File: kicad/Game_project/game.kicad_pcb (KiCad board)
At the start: 2 copper layers, 149.8 x 99.6 mm, 33 parts, among them J3 Conn_01x05_Socket, J4 Conn_01x05_Socket, J5 USB_B, J6 ISP header, U1 MAX7219, U10 HDSP-7403, U2 ATmega328P-P, U5 HDSP-7403, U6 HDSP-7403, U7 HDSP-7403, U8 HDSP-7403, U9 HDSP-7403

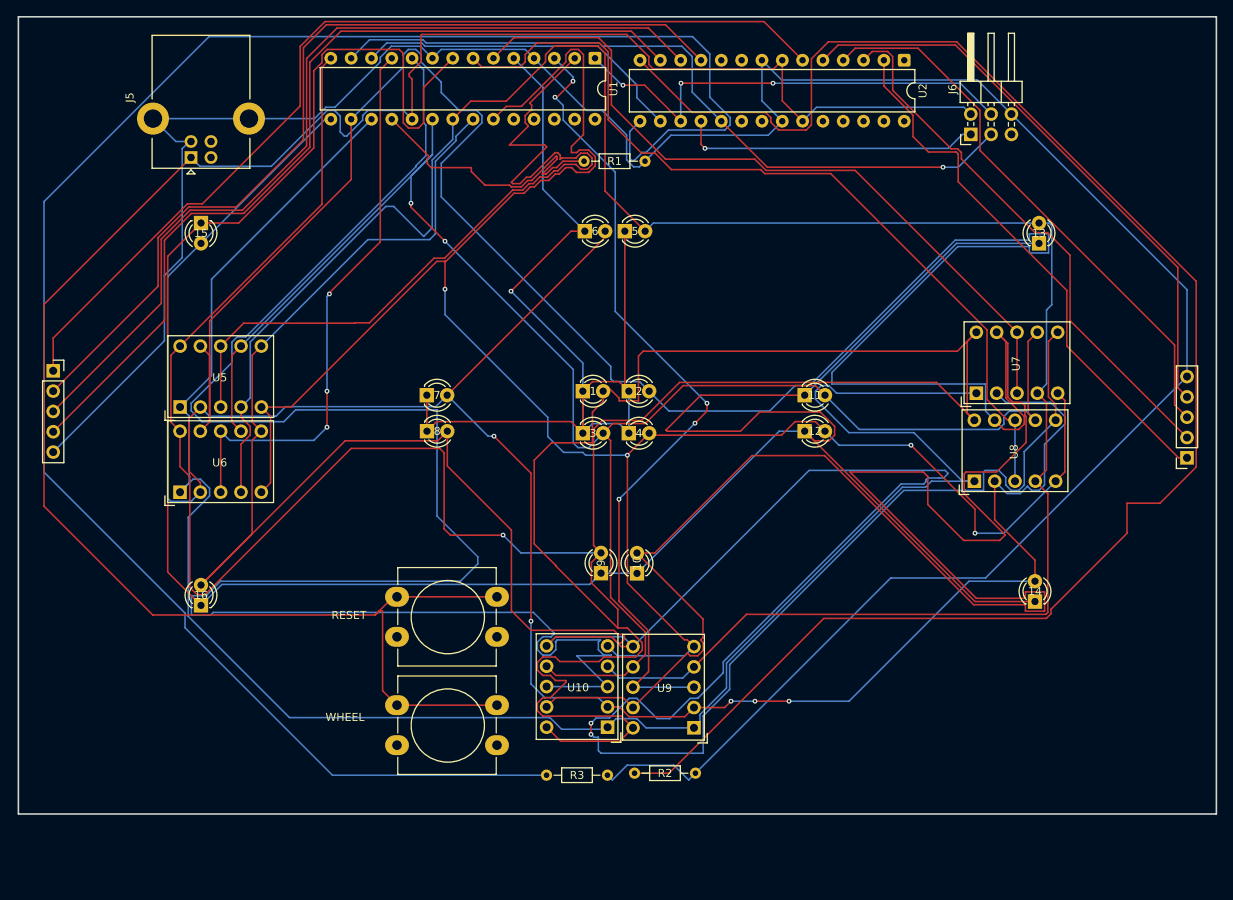
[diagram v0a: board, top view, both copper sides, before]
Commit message: orded
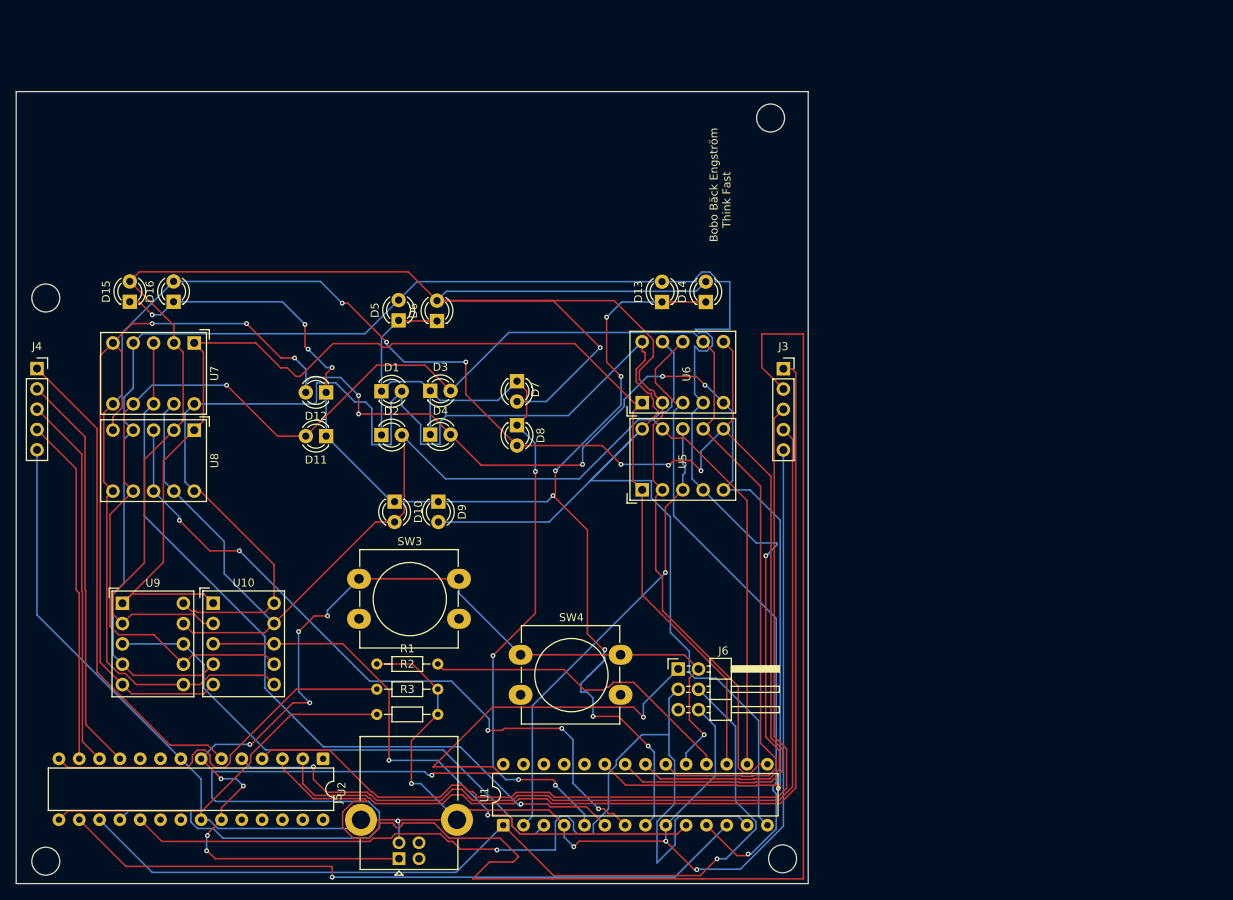
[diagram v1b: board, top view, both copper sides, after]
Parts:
- removed 1, 10, 11, 12, 13, 14, 15, 16, 2, 3, 4, 5, 6, 7, 8, 9: LED, LED_THT:LED_D3.0mm_Clear
- removed RESET, WHEEL: SW_pin12, Button_Switch_THT:SW_PUSH-12mm_Wuerth-430476085716
- added D1: LED, LED_THT:LED_D3.0mm_Clear, F.Cu at (145.6, 97.3)
- added D10: LED, LED_THT:LED_D3.0mm_Clear, F.Cu at (147.2, 111.1)
- added D11: LED, LED_THT:LED_D3.0mm_Clear, F.Cu at (138.6, 102.9)
- added D12: LED, LED_THT:LED_D3.0mm_Clear, F.Cu at (138.6, 97.4)
- added D13: LED, LED_THT:LED_D3.0mm_Clear, F.Cu at (180.6, 86.1)
- added D14: LED, LED_THT:LED_D3.0mm_Clear, F.Cu at (186.1, 86.1)
- added D15: LED, LED_THT:LED_D3.0mm_Clear, F.Cu at (114.1, 86.1)
- added D16: LED, LED_THT:LED_D3.0mm_Clear, F.Cu at (119.6, 86.1)
- added D2: LED, LED_THT:LED_D3.0mm_Clear, F.Cu at (145.6, 102.7)
- added D3: LED, LED_THT:LED_D3.0mm_Clear, F.Cu at (151.7, 97.2)
- added D4: LED, LED_THT:LED_D3.0mm_Clear, F.Cu at (151.7, 102.7)
- added D5: LED, LED_THT:LED_D3.0mm_Clear, F.Cu at (147.7, 88.4)
- added D6: LED, LED_THT:LED_D3.0mm_Clear, F.Cu at (152.5, 88.5)
- added D7: LED, LED_THT:LED_D3.0mm_Clear, F.Cu at (162.5, 96.0)
- added D8: LED, LED_THT:LED_D3.0mm_Clear, F.Cu at (162.5, 101.5)
- added D9: LED, LED_THT:LED_D3.0mm_Clear, F.Cu at (152.7, 111.1)
- added SW3: SW_pin12, Button_Switch_THT:SW_PUSH-12mm_Wuerth-430476085716, F.Cu at (142.8, 120.7)
- added SW4: SW_pin12, Button_Switch_THT:SW_PUSH-12mm_Wuerth-430476085716, F.Cu at (162.9, 130.2)
- moved U2 113.6 mm to (138.3, 143.2)
- moved U7 98.0 mm to (122.2, 91.2), turned to -90 degrees
- moved U8 97.7 mm to (122.2, 102.1), turned to -90 degrees
- moved U1 96.6 mm to (160.8, 151.5), turned to 90 degrees
- moved J5 91.4 mm to (147.8, 155.7)
- moved J6 76.2 mm to (182.7, 132.0), turned to 0 degrees
- moved U9 73.1 mm to (113.2, 123.8), turned to 0 degrees
- moved R1 71.2 mm to (145.0, 131.3), turned to 0 degrees
- moved U6 58.8 mm to (178.1, 98.7)
- moved U5 58.7 mm to (178.1, 109.6)
- moved U10 51.7 mm to (124.5, 123.7), turned to 0 degrees
- moved J3 51.7 mm to (195.8, 94.4), turned to 0 degrees
- moved R2 33.9 mm to (145.0, 134.5)
- moved R3 22.5 mm to (145.0, 137.7)
- moved J4 2.04 mm to (102.5, 94.4)
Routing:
- net /B: track 470.5 -> 175.2 mm
- net /PB1: track 235.7 -> 45.7 mm
- net /PB0: track 207.1 -> 47.7 mm
- net /DP: track 394.9 -> 239.3 mm, vias 2 -> 6
- net /DIG5: track 231.2 -> 75.5 mm, vias 0 -> 2
- net /DIG7: track 320.2 -> 169.0 mm, vias 0 -> 11
- net /A: track 387.2 -> 236.6 mm, vias 1 -> 0
- net +5V: track 266.7 -> 139.9 mm, vias 0 -> 9
- net MISO: track 37.6 -> 145.2 mm, vias 1 -> 2
- net /PD1: track 68.6 -> 174.6 mm
- net GND: track 326.0 -> 235.2 mm, vias 0 -> 5
- net /G: track 245.6 -> 162.9 mm
- net /PD7: track 110.2 -> 43.3 mm
- net /PD6: track 111.1 -> 46.9 mm
- net /PD5: track 112.1 -> 50.5 mm
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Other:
- board size 149.8 x 99.6 mm -> 99 x 99 mm
- board text added: "Bobo Bäck Engström Think Fast"
- board text removed: "12.Ta två shots och hoppa på ett ben i 10 sekunder 13.Ta en {dblquote}grenad{dblquote} (shot + öl svep direkt efter varandra) 14.Byt ut din drink mot någon annans i nästa runda 15.Drick tre klunkar ur varje annan spelares drink 16.Halsa en öl och snurra 10 varv på stället 17.Drick upp det starkaste du hittar på bordet 18.Ta en shot och försök göra en kullerbytta 19.Häll upp tre shots - drick en o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"
